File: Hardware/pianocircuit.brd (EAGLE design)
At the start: 160 x 82.2 mm, 70 parts, among them IC1 LM386M-1

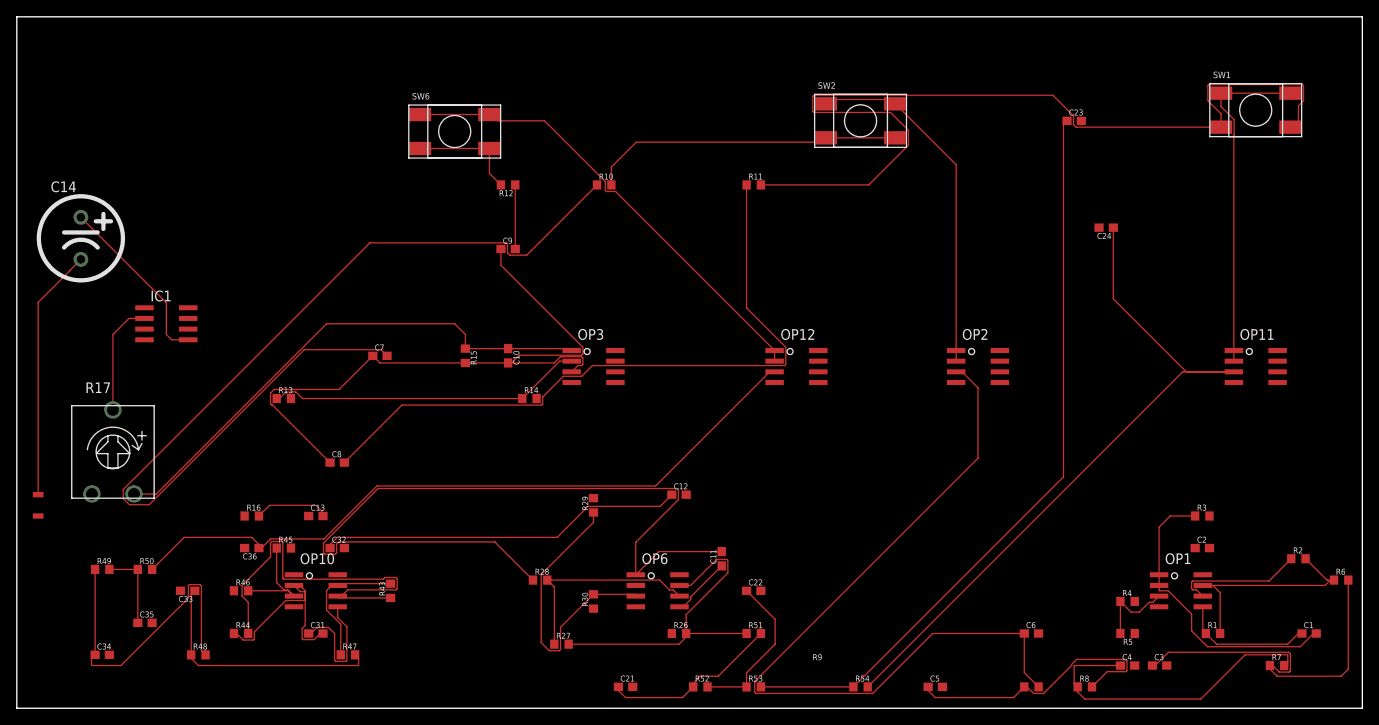
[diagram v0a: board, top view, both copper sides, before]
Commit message: Reorganizing Board
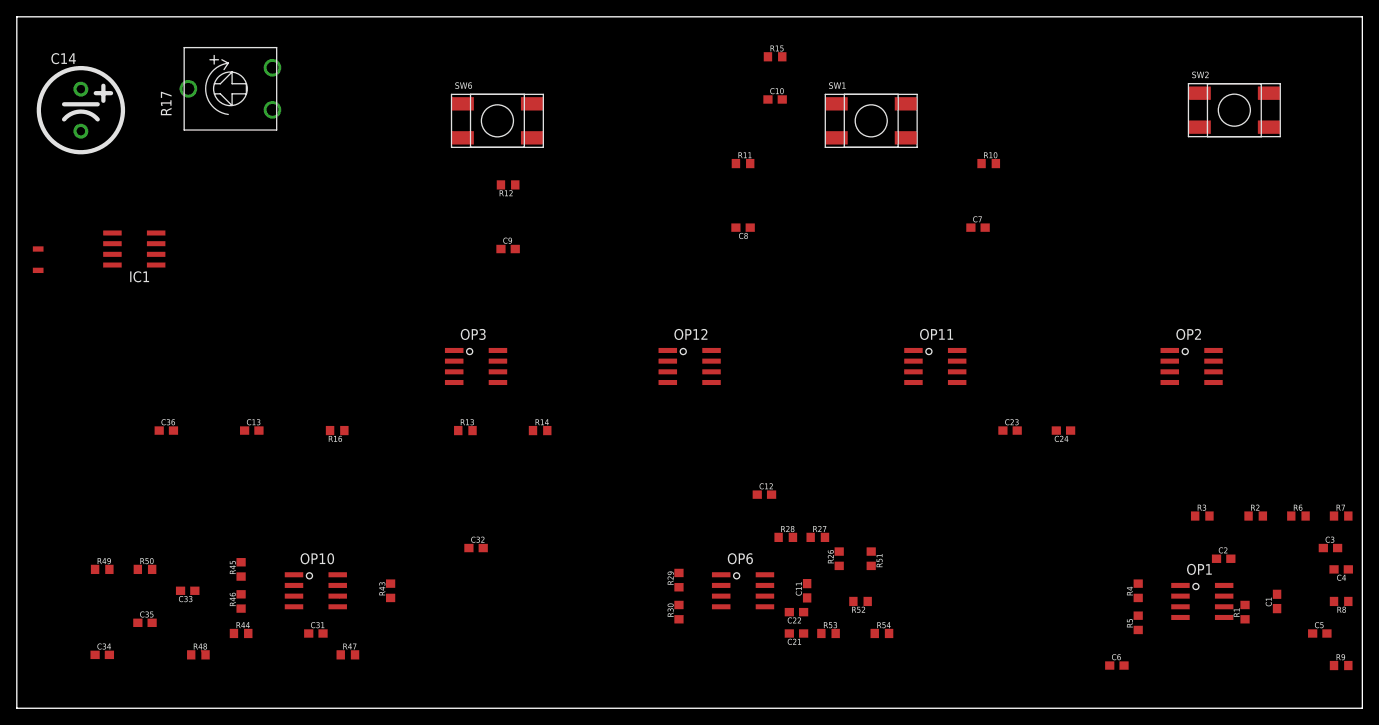
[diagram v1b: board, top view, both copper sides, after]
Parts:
- moved C7 72.7 mm to (114.3, 57.1)
- moved C8 55.8 mm to (86.4, 57.1), turned to 180 degrees
- moved R15 51.2 mm to (90.2, 77.5), turned to 0 degrees
- moved C5 46.2 mm to (154.9, 8.89)
- moved R10 45.8 mm to (115.6, 64.8)
- moved SW1 45.7 mm to (101.6, 69.8)
- moved R17 45.4 mm to (25.4, 73.7), turned to 90 degrees
- moved SW2 44.5 mm to (144.8, 71.1)
- moved C10 44.0 mm to (90.2, 72.4), turned to 0 degrees
- moved OP11 38.1 mm to (109.2, 40.6)
- moved C23 37.6 mm to (118.1, 33.0)
- moved R9 36.9 mm to (157.5, 5.08)
- moved R27 33.0 mm to (95.2, 20.3)
- moved R8 32.1 mm to (157.5, 12.7), turned to 180 degrees
- moved R28 29.6 mm to (91.4, 20.3)
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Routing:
- net N$14: track 113.9 -> 0.00 mm
- net F3: track 107.6 -> 0.00 mm
- net N$28: track 97.8 -> 0.00 mm
- net N$10: track 92.7 -> 0.00 mm
- net N$54: track 88.8 -> 0.00 mm
- net N$65: track 85.1 -> 0.00 mm
- net N$55: track 85.5 -> 1.00 mm
- net N$17: track 81.1 -> 0.00 mm
- net N$15: track 79.9 -> 0.00 mm
- net N$20: track 62.7 -> 0.30 mm
- net N$66: track 54.4 -> 0.00 mm
- net N$58: track 47.0 -> 0.30 mm
- net N$2: track 43.5 -> 0.00 mm
- net N$11: track 43.0 -> 0.00 mm
- net N$7: track 43.0 -> 0.00 mm
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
